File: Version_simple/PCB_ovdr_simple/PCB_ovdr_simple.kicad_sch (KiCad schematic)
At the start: 31 parts, among them J1 Input, J2 Output, J3 Vcc, J4 Output, U1 TL072, U2 TL072

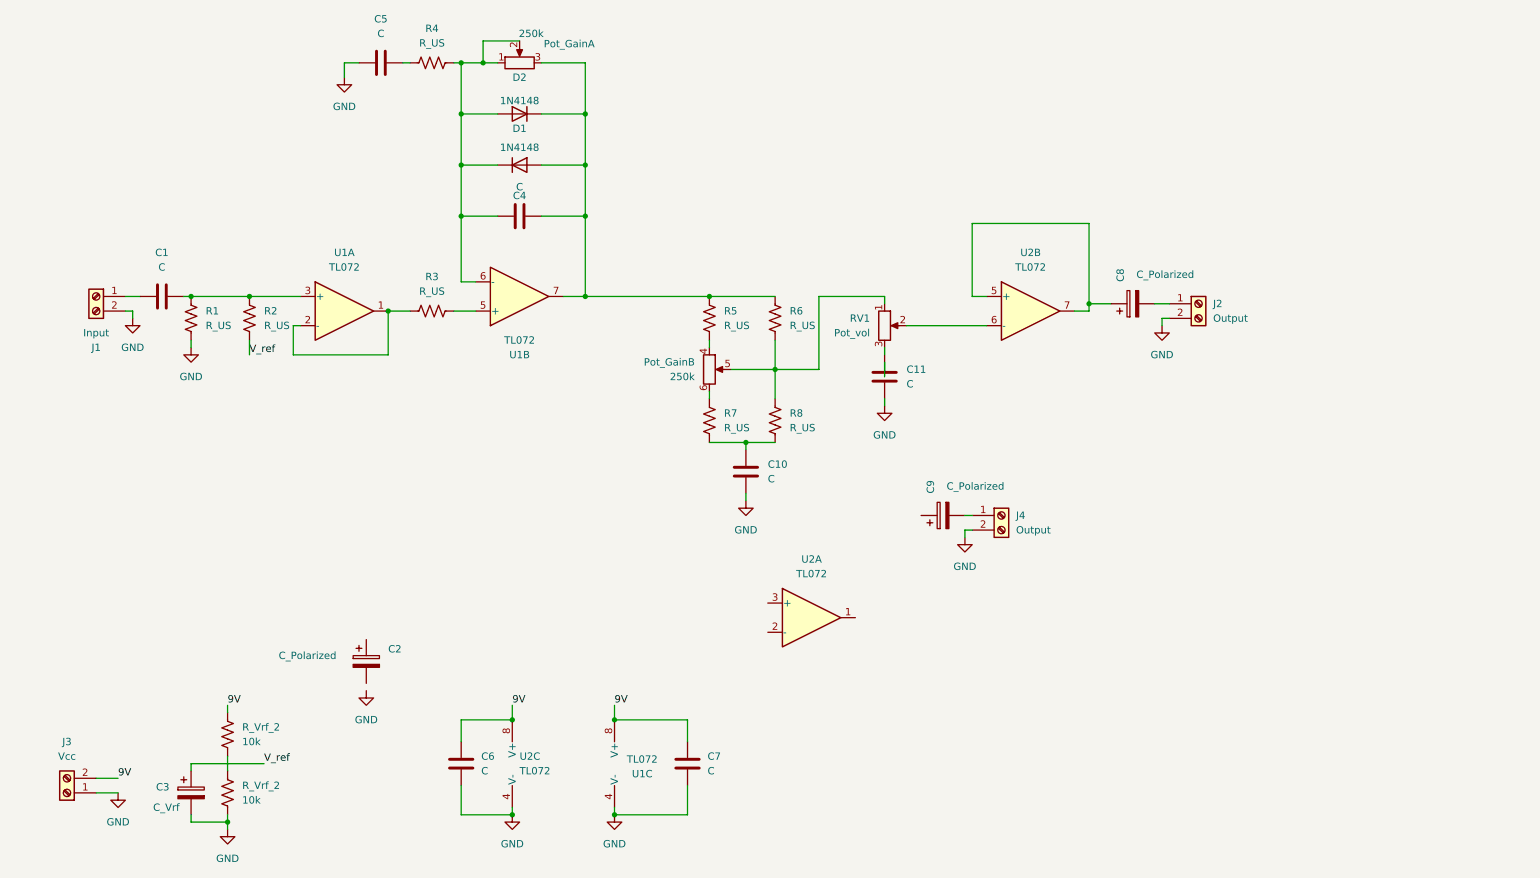
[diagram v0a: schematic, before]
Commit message: update
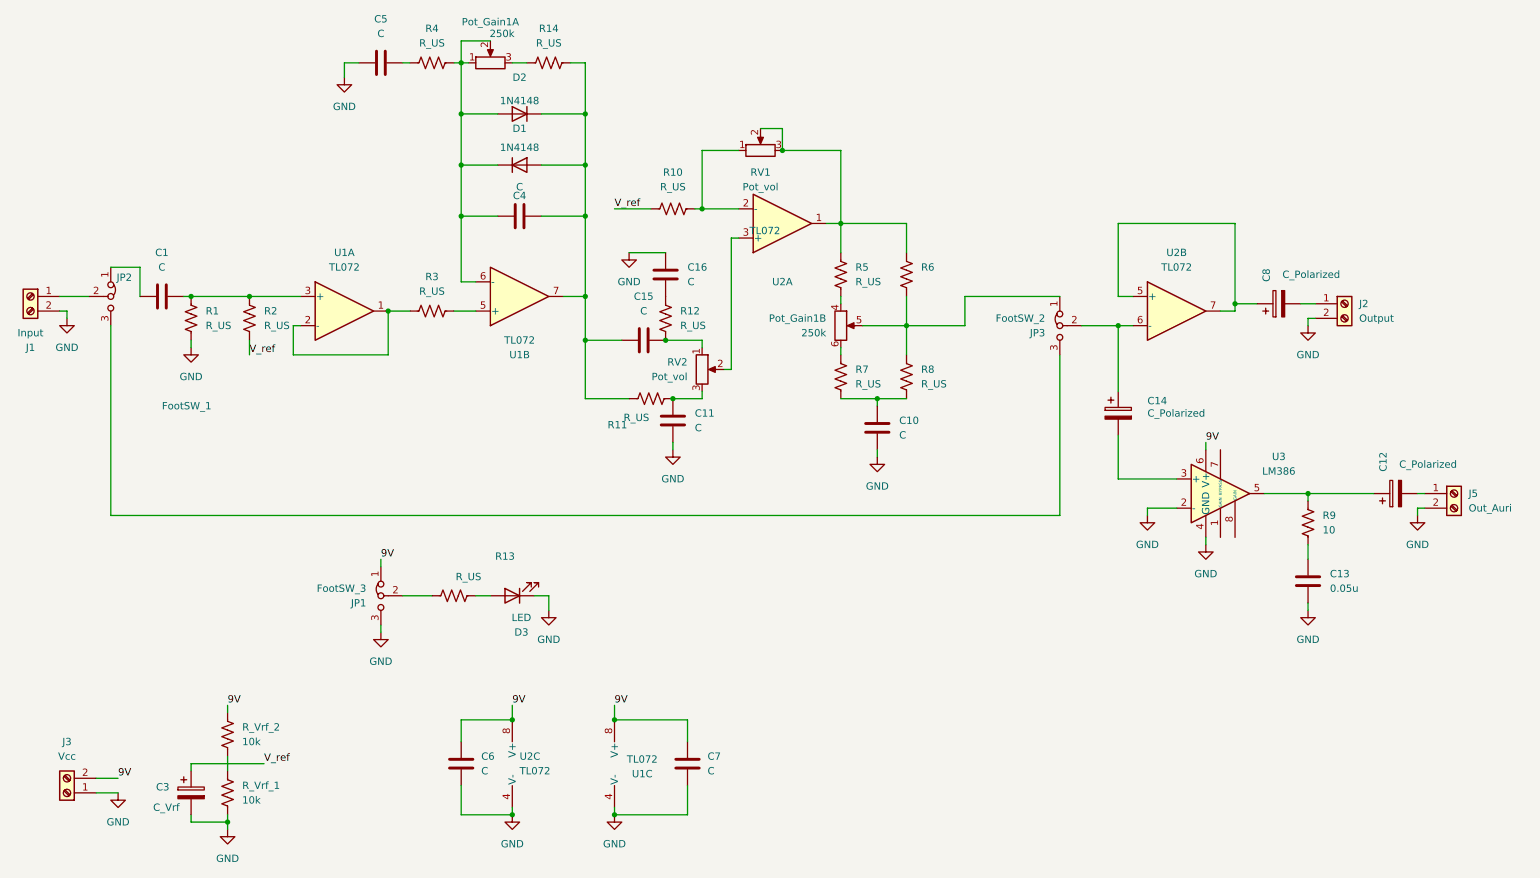
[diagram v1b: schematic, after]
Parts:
- removed C2, C9: C_Polarized, symbol Device:C_Polarized
- removed J4: Output, symbol Connector:Screw_Terminal_01x02
- added C12, C14: C_Polarized, Capacitor_THT:C_Radial_D10.0mm_H16.0mm_P5.00mm, symbol Device:C_Polarized
- added C13: 0.05u, Capacitor_THT:C_Disc_D7.0mm_W2.5mm_P5.00mm, symbol Device:C
- added C15, C16: C, Capacitor_THT:C_Disc_D7.0mm_W2.5mm_P5.00mm, symbol Device:C
- added D3: LED, Connector_PinSocket_2.54mm:PinSocket_1x02_P2.54mm_Vertical, symbol Device:LED
- added J5: Out_Auri, TerminalBlock:TerminalBlock_MaiXu_MX126-5.0-02P_1x02_P5.00mm, symbol Connector:Screw_Terminal_01x02
- added JP1: FootSW_3, Connector_PinSocket_2.54mm:PinSocket_1x03_P2.54mm_Vertical, symbol Jumper:Jumper_3_Bridged12
- added JP2: FootSW_1, Connector_PinSocket_2.54mm:PinSocket_1x03_P2.54mm_Vertical, symbol Jumper:Jumper_3_Bridged12
- added JP3: FootSW_2, Connector_PinSocket_2.54mm:PinSocket_1x03_P2.54mm_Vertical, symbol Jumper:Jumper_3_Bridged12
- added R10, R11, R12, R13, R14: R_US, Resistor_THT:R_Axial_DIN0207_L6.3mm_D2.5mm_P10.16mm_Horizontal, symbol Device:R_US
- added R9: 10, Resistor_THT:R_Axial_DIN0207_L6.3mm_D2.5mm_P10.16mm_Horizontal, symbol Device:R_US
- added RV2: Pot_vol, Connector_PinSocket_2.54mm:PinSocket_1x03_P2.54mm_Vertical, symbol Device:R_Potentiometer
- added unit 1 of U1
- added U3: LM386, Package_DIP:CERDIP-8_W7.62mm_SideBrazed_LongPads, symbol Amplifier_Audio:LM386
- C1: footprint (none) -> Capacitor_THT:C_Disc_D8.0mm_W5.0mm_P7.50mm
- C10, C11, C4, C5, C6, C7: footprint (none) -> Capacitor_THT:C_Disc_D7.0mm_W2.5mm_P5.00mm
- C3, C8: footprint (none) -> Capacitor_THT:C_Radial_D10.0mm_H16.0mm_P5.00mm
- J1, J2, J3: footprint (none) -> TerminalBlock:TerminalBlock_MaiXu_MX126-5.0-02P_1x02_P5.00mm
- Pot_Gain1: renamed from Pot_Gain; footprint (none) -> Connector_PinSocket_2.54mm:PinSocket_2x03_P2.54mm_Vertical
- R1, R2, R3, R4, R5, R6, R7, R8, R_Vrf_2: footprint (none) -> Resistor_THT:R_Axial_DIN0207_L6.3mm_D2.5mm_P10.16mm_Horizontal
- RV1: footprint (none) -> Connector_PinSocket_2.54mm:PinSocket_1x03_P2.54mm_Vertical
- R_Vrf_1: renamed from R_Vrf_2; footprint (none) -> Resistor_THT:R_Axial_DIN0207_L6.3mm_D2.5mm_P10.16mm_Horizontal
- U1, U2: footprint (none) -> Package_DIP:CERDIP-8_W7.62mm_SideBrazed_LongPads
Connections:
- net 9V: now also JP1.1 (A), U3.6 (V+)
- net GND: now also C13.1, C16.2, D3.1 (K), J5.2 (Pin_2), JP1.3 (B), U3.2 (-), U3.4 (GND)
- net V_ref: now also R10.2
- net at J1.1 (Pin_1): now also JP2.2 (C); no longer C1.1
- net at C1.2, R1.1, R2.1: now also U1.3 (+); no longer U1.3 (+)
- net at C4.2, D1.2 (A), D2.1 (K)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: now also C15.2, R11.2, R14.2; no longer Pot_Gain1.3, R5.2, R6.2
- net at Pot_Gain1.5, R6.1, R8.2: now also JP3.1 (A); no longer RV1.1
- net at U2.1: now also R5.2, R6.2, RV1.2, RV1.3
- net at U2.2 (-): now also RV1.1, R10.1
- net at U2.3 (+): now also RV2.2
- net at C11.2: now also R11.1, RV2.3; no longer RV1.3
- net at U2.6 (-): now also C14.1, JP3.2 (C); no longer RV1.2
- new net: C16.1, R12.1
- new net: C15.1, R12.2, RV2.1
- new net: C1.1, JP2.1 (A)
- new net: JP1.2 (C), R13.1
- new net: Pot_Gain1.3, R14.1
- new net: C14.2, U3.3 (+)
- new net: C12.1, R9.2, U3.5
- new net: C12.2, J5.1 (Pin_1)
- new net: R3.1, U1.1, U1.2 (-)
- new net: C13.2, R9.1
- new net: D3.2 (A), R13.2
- new net: JP2.3 (B), JP3.3 (B)
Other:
- moved on the sheet: C10, C8, J1, J2, Pot_Gain1A, Pot_Gain1B, R5, R6, R7, R8, RV1, U2A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
